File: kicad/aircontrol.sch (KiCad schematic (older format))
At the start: 10 parts, among them K1 K1, K2 K2, M1 Motor_AC, SW1 SW_Push, U1 MH-Z19, U2 NodeMCUv3-ESP8266

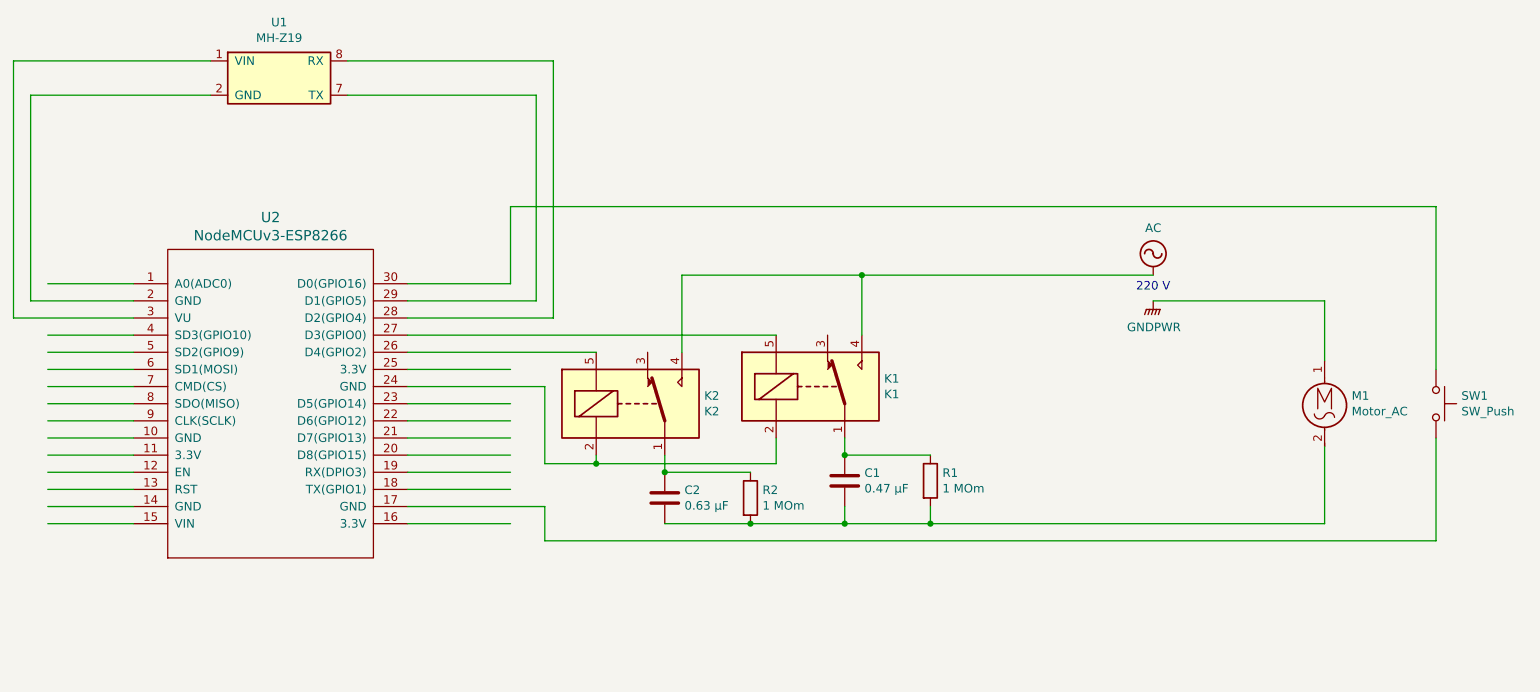
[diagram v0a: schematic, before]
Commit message: D6 pin in schema
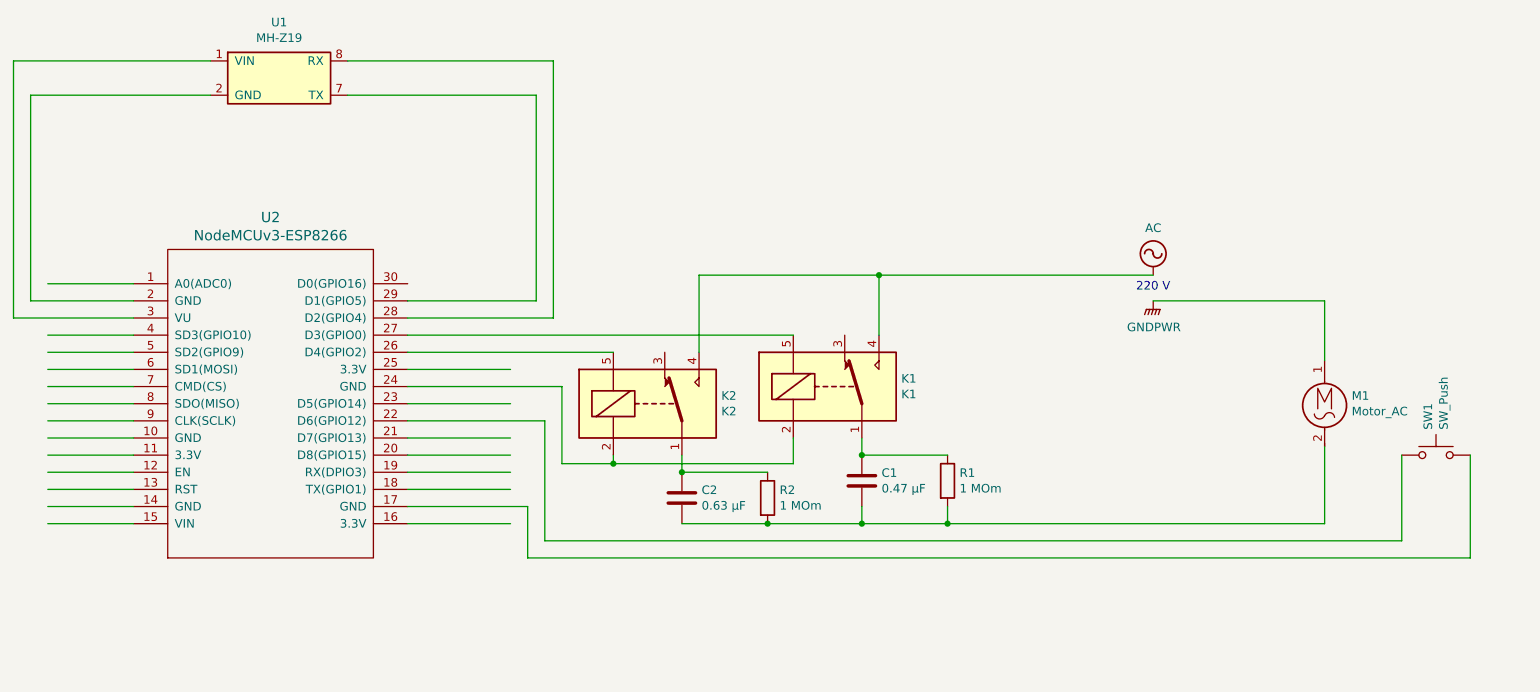
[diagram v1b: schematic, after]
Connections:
- wire segments 66 -> 65
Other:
- moved on the sheet: C1, C2, K1, K2, R1, R2, SW1
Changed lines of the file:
@@
 	2400 4350 2900 4350
 Wire Wire Line
-	4500 2950 5100 2950
-Wire Wire Line
 	4500 3450 5100 3450
 Wire Wire Line
@@
 Wire Wire Line
 	4500 3650 5100 3650
-Wire Wire Line
-	4500 3750 5100 3750
 Wire Wire Line
 	4500 3850 5100 3850
@@
 L Device:C C1
 U 1 1 604029F8
-P 7050 4100
-F 0 "C1" H 7165 4146 50  0000 L CNN
-F 1 "0.47 μF" H 7165 4055 50  0000 L CNN
-F 2 "" H 7088 3950 50  0001 C CNN
-F 3 "~" H 7050 4100 50  0001 C CNN
-	1    7050 4100
+P 7150 4100
+F 0 "C1" H 7265 4146 50  0000 L CNN
+F 1 "0.47 μF" H 7265 4055 50  0000 L CNN
+F 2 "" H 7188 3950 50  0001 C CNN
+F 3 "~" H 7150 4100 50  0001 C CNN
+	1    7150 4100
 	1    0    0    -1
 $EndComp
@@
 L Device:C C2
 U 1 1 60402AE6
-P 6000 4200
-F 0 "C2" H 6115 4246 50  0000 L CNN
-F 1 "0.63 μF" H 6115 4155 50  0000 L CNN
-F 2 "" H 6038 4050 50  0001 C CNN
-F 3 "~" H 6000 4200 50  0001 C CNN
-	1    6000 4200
+P 6100 4200
+F 0 "C2" H 6215 4246 50  0000 L CNN
+F 1 "0.63 μF" H 6215 4155 50  0000 L CNN
+F 2 "" H 6138 4050 50  0001 C CNN
+F 3 "~" H 6100 4200 50  0001 C CNN
+	1    6100 4200
 	1    0    0    -1
 $EndComp
@@
 L Relay:SANYOU_SRD_Form_C K1
 U 1 1 60402FFD
-P 6850 3550
-F 0 "K1" H 7280 3596 50  0000 L CNN
-F 1 "K1" H 7280 3505 50  0000 L CNN
-F 2 "Relay_THT:Relay_SPDT_SANYOU_SRD_Series_Form_C" H 7300 3500 50  0001 L CNN
-F 3 "http://www.sanyourelay.ca/public/products/pdf/SRD.pdf" H 6850 3550 50  0001 C CNN
-	1    6850 3550
+P 6950 3550
+F 0 "K1" H 7380 3596 50  0000 L CNN
+F 1 "K1" H 7380 3505 50  0000 L CNN
+F 2 "Relay_THT:Relay_SPDT_SANYOU_SRD_Series_Form_C" H 7400 3500 50  0001 L CNN
+F 3 "http://www.sanyourelay.ca/public/products/pdf/SRD.pdf" H 6950 3550 50  0001 C CNN
+	1    6950 3550
 	1    0    0    -1
 $EndComp
@@
 L Relay:SANYOU_SRD_Form_C K2
 U 1 1 6040311E
-P 5800 3650
-F 0 "K2" H 6230 3696 50  0000 L CNN
-F 1 "K2" H 6230 3605 50  0000 L CNN
-F 2 "Relay_THT:Relay_SPDT_SANYOU_SRD_Series_Form_C" H 6250 3600 50  0001 L CNN
-F 3 "http://www.sanyourelay.ca/public/products/pdf/SRD.pdf" H 5800 3650 50  0001 C CNN
-	1    5800 3650
-	1    0    0    -1
-$EndComp
-Wire Wire Line
-	4500 3250 6650 3250
-Wire Wire Line
-	4500 3350 5600 3350
+P 5900 3650
+F 0 "K2" H 6330 3696 50  0000 L CNN
+F 1 "K2" H 6330 3605 50  0000 L CNN
+F 2 "Relay_THT:Relay_SPDT_SANYOU_SRD_Series_Form_C" H 6350 3600 50  0001 L CNN
+F 3 "http://www.sanyourelay.ca/public/products/pdf/SRD.pdf" H 5900 3650 50  0001 C CNN
+	1    5900 3650
+	1    0    0    -1
+$EndComp
 $Comp
 L Device:R R1
 U 1 1 60409148
-P 7550 4100
-F 0 "R1" H 7620 4146 50  0000 L CNN
-F 1 "1 MOm" H 7620 4055 50  0000 L CNN
-F 2 "" V 7480 4100 50  0001 C CNN
-F 3 "~" H 7550 4100 50  0001 C CNN
-	1    7550 4100
+P 7650 4100
+F 0 "R1" H 7720 4146 50  0000 L CNN
+F 1 "1 MOm" H 7720 4055 50  0000 L CNN
+F 2 "" V 7580 4100 50  0001 C CNN
+F 3 "~" H 7650 4100 50  0001 C CNN
+	1    7650 4100
 	1    0    0    -1
 $EndComp
@@
 L Device:R R2
 U 1 1 60409274
-P 6500 4200
-F 0 "R2" H 6570 4246 50  0000 L CNN
-F 1 "1 MOm" H 6570 4155 50  0000 L CNN
-F 2 "" V 6430 4200 50  0001 C CNN
-F 3 "~" H 6500 4200 50  0001 C CNN
-	1    6500 4200
+P 6600 4200
+F 0 "R2" H 6670 4246 50  0000 L CNN
+F 1 "1 MOm" H 6670 4155 50  0000 L CNN
+F 2 "" V 6530 4200 50  0001 C CNN
+F 3 "~" H 6600 4200 50  0001 C CNN
+	1    6600 4200
 	1    0    0    -1
 $EndComp
@@
 220 V
 Wire Wire Line
-	8850 2900 7150 2900
-Wire Wire Line
-	6100 2900 6100 3350
-Wire Wire Line
-	7150 3250 7150 2900
-Connection ~ 7150 2900
-Wire Wire Line
-	7150 2900 6100 2900
-Wire Wire Line
-	7050 4250 7050 4350
-Connection ~ 7050 4350
-Wire Wire Line
-	7050 4350 7550 4350
+	8850 2900 7250 2900
+Wire Wire Line
+	6200 2900 6200 3350
+Wire Wire Line
+	7250 3250 7250 2900
+Wire Wire Line
+	7150 4250 7150 4350
+Connection ~ 7150 4350
+Wire Wire Line
+	7150 4350 7650 4350
 Wire Wire Line
 	8850 3050 9850 3050
@@
 	9850 3050 9850 3400
 Wire Wire Line
-	5600 4000 5300 4000
-Wire Wire Line
-	4500 3550 5300 3550
-Wire Wire Line
-	7050 3850 7050 3950
-Connection ~ 7050 3950
-Wire Wire Line
-	6000 4050 6000 3950
-Connection ~ 6000 4050
+	5700 4000 5400 4000
+Wire Wire Line
+	7150 3850 7150 3950
+Connection ~ 7150 3950
+Wire Wire Line
+	6100 4050 6100 3950
+Connection ~ 6100 4050
 Wire Wire Line
 	9850 3900 9850 4350
 Wire Wire Line
-	6650 4000 5600 4000
-Wire Wire Line
-	5600 4000 5600 3950
-Wire Wire Line
-	6650 3850 6650 4000
-Connection ~ 5600 4000
-Wire Wire Line
-	5300 3550 5300 4000
+	6750 4000 5700 4000
+Wire Wire Line
+	5700 4000 5700 3950
+Wire Wire Line
+	6750 3850 6750 4000
+Connection ~ 5700 4000
 $Comp
 L aircontrol-rescue:MH-Z19 U1
@@
 L Switch:SW_Push SW1
 U 1 1 604378ED
-P 10500 3650
-F 0 "SW1" V 10454 3798 50  0000 L CNN
-F 1 "SW_Push" V 10545 3798 50  0000 L CNN
-F 2 "" H 10500 3850 50  0001 C CNN
-F 3 "" H 10500 3850 50  0001 C CNN
-	1    10500 3650
-	0    1    1    0
-$EndComp
-Wire Wire Line
-	10500 3450 10500 2500
-Wire Wire Line
-	10500 2500 5100 2500
-Wire Wire Line
-	5100 2500 5100 2950
-Wire Wire Line
-	10500 3850 10500 4450
-Wire Wire Line
-	10500 4450 5300 4450
-Wire Wire Line
-	5300 4450 5300 4250
-Wire Wire Line
-	4500 4250 5300 4250
-Wire Wire Line
-	6000 4350 6500 4350
-Connection ~ 6500 4350
-Wire Wire Line
-	6500 4350 7050 4350
-Wire Wire Line
-	6000 4050 6500 4050
-Wire Wire Line
-	7050 3950 7550 3950
-Wire Wire Line
-	7550 4250 7550 4350
-Connection ~ 7550 4350
-Wire Wire Line
-	7550 4350 9850 4350
+P 10500 3950
+F 0 "SW1" V 10454 4098 50  0000 L CNN
+F 1 "SW_Push" V 10545 4098 50  0000 L CNN
+F 2 "" H 10500 4150 50  0001 C CNN
+F 3 "" H 10500 4150 50  0001 C CNN
+	1    10500 3950
+	1    0    0    -1
+$EndComp
+Wire Wire Line
+	6100 4350 6600 4350
+Connection ~ 6600 4350
+Wire Wire Line
+	6600 4350 7150 4350
+Wire Wire Line
+	6100 4050 6600 4050
+Wire Wire Line
+	7150 3950 7650 3950
+Wire Wire Line
+	7650 4250 7650 4350
+Connection ~ 7650 4350
+Wire Wire Line
+	7650 4350 9850 4350
+Wire Wire Line
+	5300 3750 5300 4450
+Wire Wire Line
+	10300 4450 10300 3950
+Wire Wire Line
+	10700 3950 10700 4550
+Wire Wire Line
+	5200 4550 5200 4250
+Connection ~ 7250 2900
+Wire Wire Line
+	6200 2900 7250 2900
+Wire Wire Line
+	4500 3250 6750 3250
+Wire Wire Line
+	4500 3350 5700 3350
+Wire Wire Line
+	5400 4000 5400 3550
+Wire Wire Line
+	4500 3550 5400 3550
+Wire Wire Line
+	5300 4450 10300 4450
+Wire Wire Line
+	4500 3750 5300 3750
+Wire Wire Line
+	5200 4550 10700 4550
+Wire Wire Line
+	4500 4250 5200 4250
 $EndSCHEMATC

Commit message: mhz19.yaml-coded pins to kicad: mh-z19 to rx-tx, relays to gpio12-13, button to 14
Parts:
- K1, K2: symbol Relay:SANYOU_SRD_Form_C -> aircontrol-rescue:SANYOU_SRD_Form_C-Relay
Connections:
- wire segments 65 -> 62
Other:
- moved on the sheet: C1, C2, K1, K2, M1, R1, R2, SW1, U1
